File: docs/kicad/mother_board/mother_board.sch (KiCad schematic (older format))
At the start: 14 parts, among them J1 EXPR, J2 TFT_CONTROL, J3 TFT_DATA, J4 SERIAL, J5 LEDS, J6 ROTARY12, J7 ROTARY34, J8 SW_OUT, J9 SW_IN, U1 myTeensy3.6

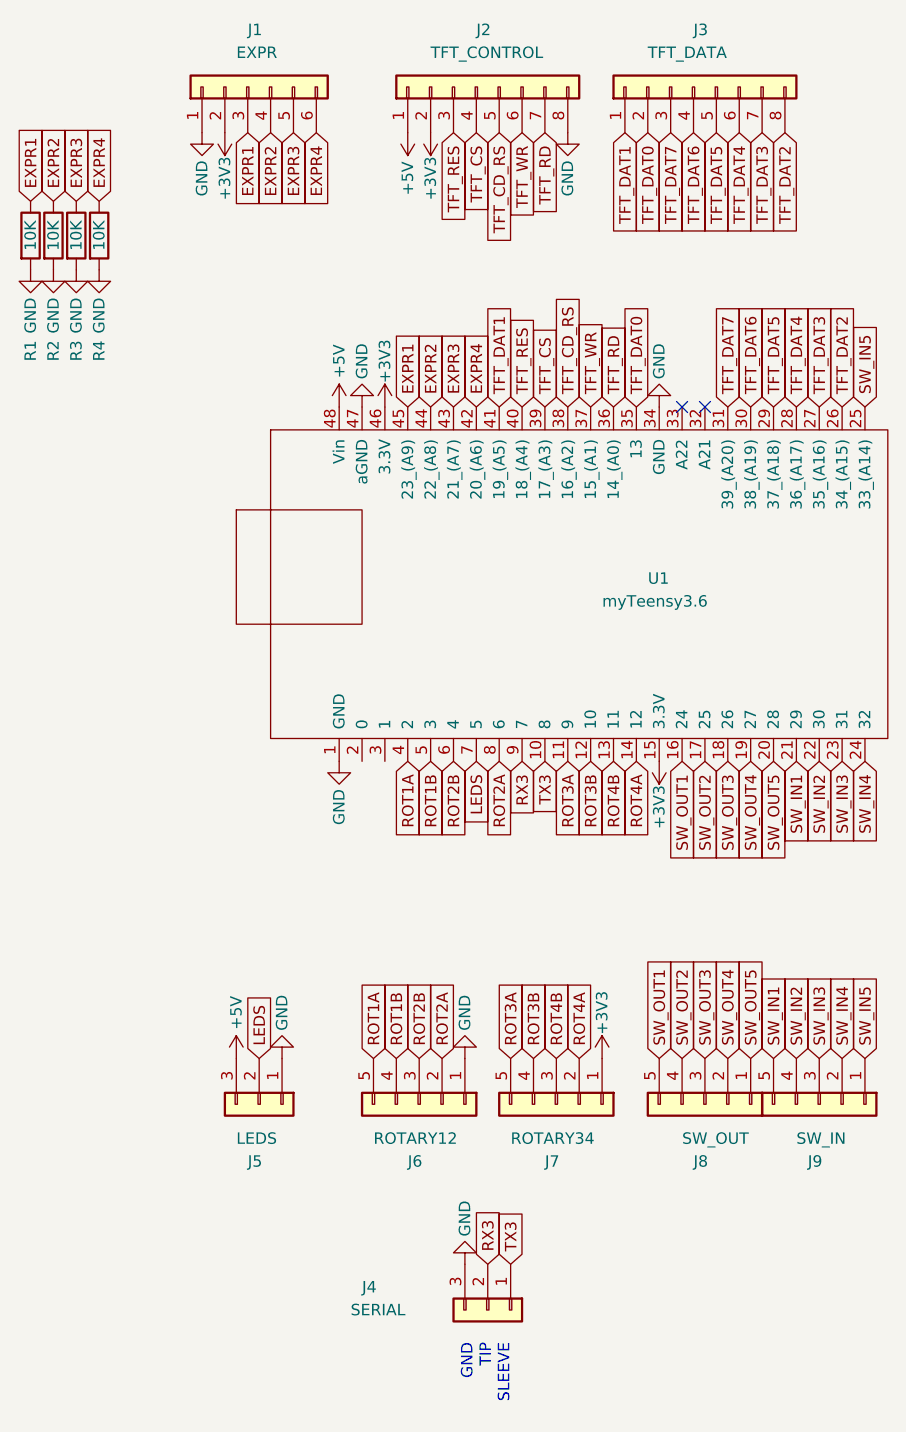
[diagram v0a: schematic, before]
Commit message: start MAKE NEW motherboard and display_connector FOR olds TeensyExprssion box with TE2 code
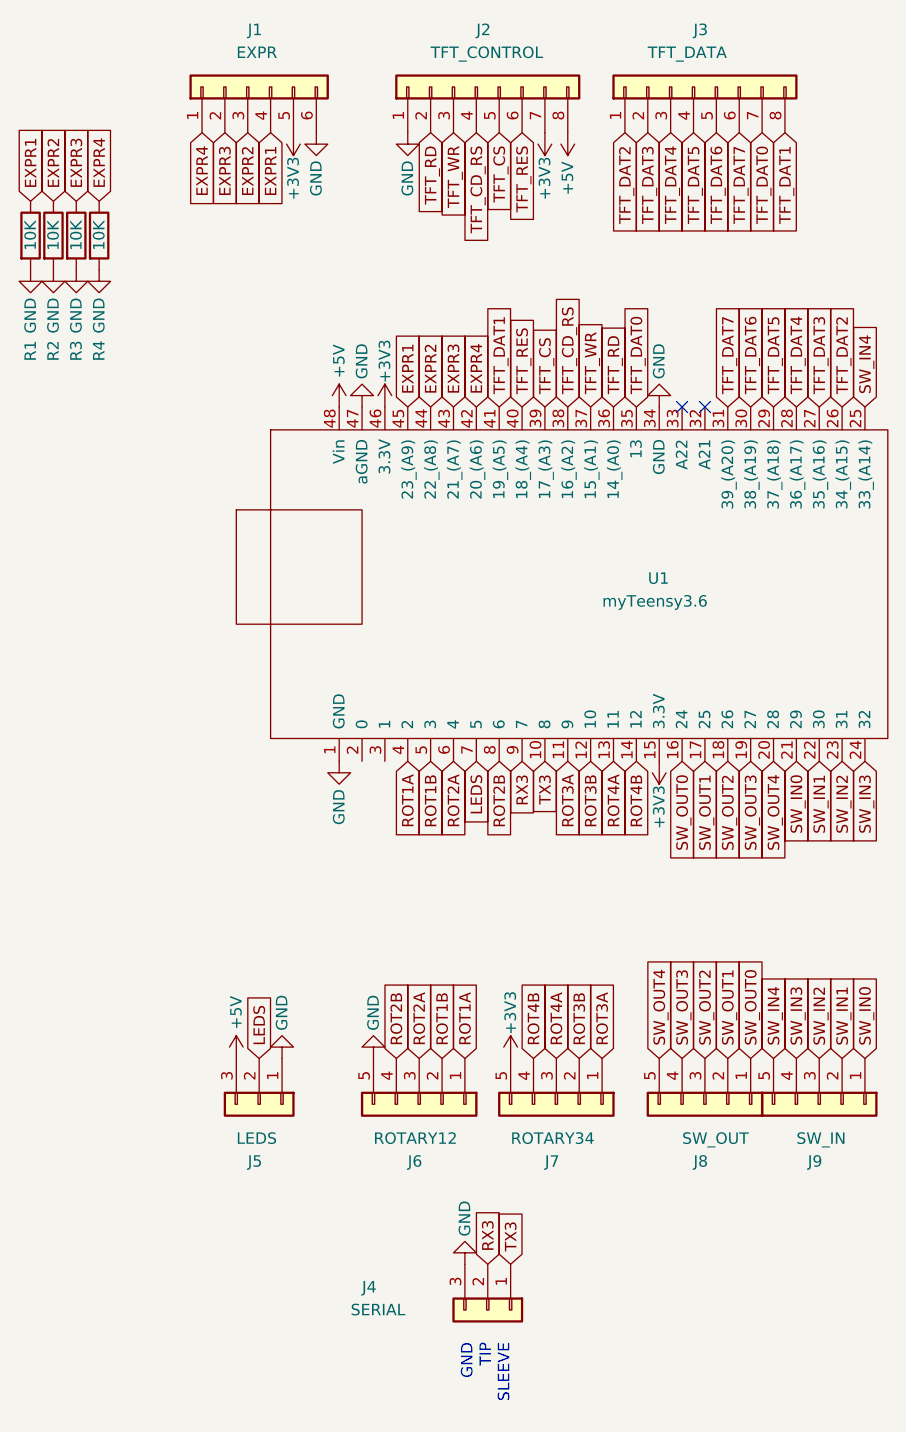
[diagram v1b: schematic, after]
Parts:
- J1: footprint 0_my_footprints:myJSTx06 -> 0_my_footprints:myPinSocket_1x06
- J4, J5: footprint 0_my_footprints:myJSTx03 -> 0_my_footprints:myPinSocket_1x03
- J6, J7, J8, J9: footprint 0_my_footprints:myJSTx05 -> 0_my_footprints:myPinSocket_1x05
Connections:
- net +3V3: now also J1.5 (Pin_5), J2.7 (Pin_7), J7.5 (Pin_5); no longer J1.2 (Pin_2), J2.2 (Pin_2), J7.1 (Pin_1)
- net +5V: now also J2.8 (Pin_8); no longer J2.1 (Pin_1)
- net EXPR1: now also J1.4 (Pin_4); no longer J1.3 (Pin_3)
- net EXPR2: now also J1.3 (Pin_3); no longer J1.4 (Pin_4)
- net EXPR3: now also J1.2 (Pin_2); no longer J1.5 (Pin_5)
- net EXPR4: now also J1.1 (Pin_1); no longer J1.6 (Pin_6)
- net GND: now also J1.6 (Pin_6), J2.1 (Pin_1), J6.5 (Pin_5); no longer J1.1 (Pin_1), J2.8 (Pin_8), J6.1 (Pin_1)
- net ROT1A: now also J6.1 (Pin_1); no longer J6.5 (Pin_5)
- net ROT1B: now also J6.2 (Pin_2); no longer J6.4 (Pin_4)
- net ROT2A: now also J6.3 (Pin_3), U1.6 (4); no longer J6.2 (Pin_2), U1.8 (6)
- net ROT2B: now also J6.4 (Pin_4), U1.8 (6); no longer J6.3 (Pin_3), U1.6 (4)
- net ROT3A: now also J7.1 (Pin_1); no longer J7.5 (Pin_5)
- net ROT3B: now also J7.2 (Pin_2); no longer J7.4 (Pin_4)
- net ROT4A: now also J7.3 (Pin_3), U1.13 (11); no longer J7.2 (Pin_2), U1.14 (12)
- net ROT4B: now also J7.4 (Pin_4), U1.14 (12); no longer J7.3 (Pin_3), U1.13 (11)
- net SW_IN1: now also J9.2 (Pin_2), U1.22 (30); no longer J9.5 (Pin_5), U1.21 (29)
- net SW_IN2: now also J9.3 (Pin_3), U1.23 (31); no longer J9.4 (Pin_4), U1.22 (30)
- net SW_IN3: now also J9.4 (Pin_4), U1.24 (32); no longer J9.3 (Pin_3), U1.23 (31)
- net SW_IN4: now also J9.5 (Pin_5), U1.25 (33_(A14)); no longer J9.2 (Pin_2), U1.24 (32)
- net SW_OUT1: now also J8.2 (Pin_2), U1.17 (25); no longer J8.5 (Pin_5), U1.16 (24)
- net SW_OUT2: now also J8.3 (Pin_3), U1.18 (26); no longer J8.4 (Pin_4), U1.17 (25)
- net SW_OUT3: now also J8.4 (Pin_4), U1.19 (27); no longer J8.3 (Pin_3), U1.18 (26)
- net SW_OUT4: now also J8.5 (Pin_5), U1.20 (28); no longer J8.2 (Pin_2), U1.19 (27)
- net TFT_CD_RS: now also J2.4 (Pin_4); no longer J2.5 (Pin_5)
- net TFT_CS: now also J2.5 (Pin_5); no longer J2.4 (Pin_4)
- net TFT_DAT0: now also J3.7 (Pin_7); no longer J3.2 (Pin_2)
- net TFT_DAT1: now also J3.8 (Pin_8); no longer J3.1 (Pin_1)
- net TFT_DAT2: now also J3.1 (Pin_1); no longer J3.8 (Pin_8)
- net TFT_DAT3: now also J3.2 (Pin_2); no longer J3.7 (Pin_7)
- net TFT_DAT4: now also J3.3 (Pin_3); no longer J3.6 (Pin_6)
- net TFT_DAT5: now also J3.4 (Pin_4); no longer J3.5 (Pin_5)
- net TFT_DAT6: now also J3.5 (Pin_5); no longer J3.4 (Pin_4)
- net TFT_DAT7: now also J3.6 (Pin_6); no longer J3.3 (Pin_3)
- net TFT_RD: now also J2.2 (Pin_2); no longer J2.7 (Pin_7)
- net TFT_RES: now also J2.6 (Pin_6); no longer J2.3 (Pin_3)
- net TFT_WR: now also J2.3 (Pin_3); no longer J2.6 (Pin_6)
- net SW_IN5 renamed SW_IN0
- net SW_IN0: now also U1.21 (29); no longer U1.25 (33_(A14))
- net SW_OUT5 renamed SW_OUT0
- net SW_OUT0: now also U1.16 (24); no longer U1.20 (28)
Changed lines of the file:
@@
 F 0 "J5" V 4250 5700 50  0000 L CNN
 F 1 "LEDS" V 4150 5650 50  0000 L CNN
-F 2 "0_my_footprints:myJSTx03" H 4000 5750 50  0001 C CNN
+F 2 "0_my_footprints:myPinSocket_1x03" H 4000 5750 50  0001 C CNN
 F 3 "~" H 4000 5750 50  0001 C CNN
 	1    4000 5750
@@
 F 0 "J6" V 4950 5700 50  0000 L CNN
 F 1 "ROTARY12" V 4850 5550 50  0000 L CNN
-F 2 "0_my_footprints:myJSTx05" H 4700 5750 50  0001 C CNN
+F 2 "0_my_footprints:myPinSocket_1x05" H 4700 5750 50  0001 C CNN
 F 3 "~" H 4700 5750 50  0001 C CNN
 	1    4700 5750
@@
 F 0 "J1" V 4200 1300 50  0000 R CNN
 F 1 "EXPR" V 4100 1350 50  0000 R CNN
-F 2 "0_my_footprints:myJSTx06" H 3950 1300 50  0001 C CNN
+F 2 "0_my_footprints:myPinSocket_1x06" H 3950 1300 50  0001 C CNN
 F 3 "~" H 3950 1300 50  0001 C CNN
 	1    3950 1300
@@
 F 0 "J7" V 5550 5700 50  0000 L CNN
 F 1 "ROTARY34" V 5450 5550 50  0000 L CNN
-F 2 "0_my_footprints:myJSTx05" H 5300 5750 50  0001 C CNN
+F 2 "0_my_footprints:myPinSocket_1x05" H 5300 5750 50  0001 C CNN
 F 3 "~" H 5300 5750 50  0001 C CNN
 	1    5300 5750
@@
 F 0 "J8" V 6200 5700 50  0000 L CNN
 F 1 "SW_OUT" V 6100 5650 50  0000 L CNN
-F 2 "0_my_footprints:myJSTx05" H 5950 5750 50  0001 C CNN
+F 2 "0_my_footprints:myPinSocket_1x05" H 5950 5750 50  0001 C CNN
 F 3 "~" H 5950 5750 50  0001 C CNN
 	1    5950 5750
@@
 F 0 "J9" V 6700 5700 50  0000 L CNN
 F 1 "SW_IN" V 6600 5650 50  0000 L CNN
-F 2 "0_my_footprints:myJSTx05" H 6450 5750 50  0001 C CNN
+F 2 "0_my_footprints:myPinSocket_1x05" H 6450 5750 50  0001 C CNN
 F 3 "~" H 6450 5750 50  0001 C CNN
 	1    6450 5750
@@
 F 0 "J4" V 4900 6100 50  0000 L CNN
 F 1 "SERIAL" V 5000 6050 50  0000 L CNN
-F 2 "0_my_footprints:myJSTx03" H 5000 6650 50  0001 C CNN
+F 2 "0_my_footprints:myPinSocket_1x03" H 5000 6650 50  0001 C CNN
 F 3 "~" H 5000 6650 50  0001 C CNN
 	1    5000 6650
@@
 L power:+3V3 #PWR016
 U 1 1 64C9FDB5
-P 5500 5550
-F 0 "#PWR016" H 5500 5400 50  0001 C CNN
-F 1 "+3V3" V 5500 5750 50  0000 C CNN
-F 2 "" H 5500 5550 50  0001 C CNN
-F 3 "" H 5500 5550 50  0001 C CNN
-	1    5500 5550
+P 5100 5550
+F 0 "#PWR016" H 5100 5400 50  0001 C CNN
+F 1 "+3V3" V 5100 5750 50  0000 C CNN
+F 2 "" H 5100 5550 50  0001 C CNN
+F 3 "" H 5100 5550 50  0001 C CNN
+	1    5100 5550
 	1    0    0    -1
 $EndComp
@@
 L power:GND #PWR015
 U 1 1 64CA12B5
-P 4900 5550
-F 0 "#PWR015" H 4900 5300 50  0001 C CNN
-F 1 "GND" V 4900 5350 50  0000 C CNN
-F 2 "" H 4900 5550 50  0001 C CNN
-F 3 "" H 4900 5550 50  0001 C CNN
-	1    4900 5550
+P 4500 5550
+F 0 "#PWR015" H 4500 5300 50  0001 C CNN
+F 1 "GND" V 4500 5350 50  0000 C CNN
+F 2 "" H 4500 5550 50  0001 C CNN
+F 3 "" H 4500 5550 50  0001 C CNN
+	1    4500 5550
 	-1   0    0    1
 $EndComp
@@
 	-1   0    0    1
 $EndComp
-Text GLabel 4950 4250 3    50   Input ~ 0
-LEDS
 Text GLabel 4650 4250 3    50   Input ~ 0
 ROT1A
@@
 ROT1B
 Text GLabel 4850 4250 3    50   Input ~ 0
-ROT2B
-Text GLabel 5050 4250 3    50   Input ~ 0
 ROT2A
 Text GLabel 5150 4250 3    50   Input ~ 0
@@
 Text GLabel 5450 4250 3    50   Input ~ 0
 ROT3B
+Text GLabel 5650 4250 3    50   Input ~ 0
+ROT4B
 Text GLabel 5550 4250 3    50   Input ~ 0
+ROT4A
+Text GLabel 4900 5550 1    50   Input ~ 0
+ROT1A
+Text GLabel 4800 5550 1    50   Input ~ 0
+ROT1B
+Text GLabel 4600 5550 1    50   Input ~ 0
+ROT2B
+Text GLabel 4700 5550 1    50   Input ~ 0
+ROT2A
+Text GLabel 5500 5550 1    50   Input ~ 0
+ROT3A
+Text GLabel 5400 5550 1    50   Input ~ 0
+ROT3B
+Text GLabel 5200 5550 1    50   Input ~ 0
 ROT4B
-Text GLabel 5650 4250 3    50   Input ~ 0
-ROT4A
-Text GLabel 4500 5550 1    50   Input ~ 0
-ROT1A
-Text GLabel 4600 5550 1    50   Input ~ 0
-ROT1B
-Text GLabel 4700 5550 1    50   Input ~ 0
-ROT2B
-Text GLabel 4800 5550 1    50   Input ~ 0
-ROT2A
-Text GLabel 5100 5550 1    50   Input ~ 0
-ROT3A
-Text GLabel 5200 5550 1    50   Input ~ 0
-ROT3B
 Text GLabel 5300 5550 1    50   Input ~ 0
-ROT4B
-Text GLabel 5400 5550 1    50   Input ~ 0
 ROT4A
 Text GLabel 5850 4250 3    50   Input ~ 0
+SW_OUT0
+Text GLabel 5950 4250 3    50   Input ~ 0
 SW_OUT1
-Text GLabel 5950 4250 3    50   Input ~ 0
+Text GLabel 6050 4250 3    50   Input ~ 0
 SW_OUT2
-Text GLabel 6050 4250 3    50   Input ~ 0
+Text GLabel 6150 4250 3    50   Input ~ 0
 SW_OUT3
-Text GLabel 6150 4250 3    50   Input ~ 0
+Text GLabel 6250 4250 3    50   Input ~ 0
 SW_OUT4
-Text GLabel 6250 4250 3    50   Input ~ 0
-SW_OUT5
 Text GLabel 6350 4250 3    50   Input ~ 0
+SW_IN0
+Text GLabel 6450 4250 3    50   Input ~ 0
 SW_IN1
-Text GLabel 6450 4250 3    50   Input ~ 0
+Text GLabel 6550 4250 3    50   Input ~ 0
 SW_IN2
-Text GLabel 6550 4250 3    50   Input ~ 0
+Text GLabel 6650 4250 3    50   Input ~ 0
 SW_IN3
-Text GLabel 6650 4250 3    50   Input ~ 0
+Text GLabel 6650 2700 1    50   Input ~ 0
 SW_IN4
-Text GLabel 6650 2700 1    50   Input ~ 0
-SW_IN5
+Text GLabel 6050 5550 1    50   Input ~ 0
+SW_OUT1
+Text GLabel 5950 5550 1    50   Input ~ 0
+SW_OUT2
+Text GLabel 5850 5550 1    50   Input ~ 0
+SW_OUT3
 Text GLabel 5750 5550 1    50   Input ~ 0
-SW_OUT1
-Text GLabel 5850 5550 1    50   Input ~ 0
-SW_OUT2
-Text GLabel 5950 5550 1    50   Input ~ 0
-SW_OUT3
-Text GLabel 6050 5550 1    50   Input ~ 0
 SW_OUT4
 Text GLabel 6150 5550 1    50   Input ~ 0
-SW_OUT5
+SW_OUT0
+Text GLabel 6550 5550 1    50   Input ~ 0
+SW_IN1
+Text GLabel 6450 5550 1    50   Input ~ 0
+SW_IN2
+Text GLabel 6350 5550 1    50   Input ~ 0
+SW_IN3
 Text GLabel 6250 5550 1    50   Input ~ 0
-SW_IN1
-Text GLabel 6350 5550 1    50   Input ~ 0
-SW_IN2
-Text GLabel 6450 5550 1    50   Input ~ 0
-SW_IN3
-Text GLabel 6550 5550 1    50   Input ~ 0
 SW_IN4
 Text GLabel 6650 5550 1    50   Input ~ 0
-SW_IN5
+SW_IN0
 $Comp
 L power:GND #PWR01
 U 1 1 64CFCC09
-P 3750 1500
-F 0 "#PWR01" H 3750 1250 50  0001 C CNN
-F 1 "GND" V 3750 1300 50  0000 C CNN
-F 2 "" H 3750 1500 50  0001 C CNN
-F 3 "" H 3750 1500 50  0001 C CNN
-	1    3750 1500
-	1    0    0    -1
+P 4250 1500
+F 0 "#PWR01" H 4250 1250 50  0001 C CNN
+F 1 "GND" V 4250 1300 50  0000 C CNN
+F 2 "" H 4250 1500 50  0001 C CNN
+F 3 "" H 4250 1500 50  0001 C CNN
+	1    4250 1500
+	-1   0    0    -1
 $EndComp
 $Comp
@@
 	1    0    0    -1
 $EndComp
+Text GLabel 4050 1500 3    50   Input ~ 0
+EXPR1
 Text GLabel 3950 1500 3    50   Input ~ 0
-EXPR1
-Text GLabel 4050 1500 3    50   Input ~ 0
 EXPR2
-Text GLabel 4150 1500 3    50   Input ~ 0
+Text GLabel 3850 1500 3    50   Input ~ 0
 EXPR3
-Text GLabel 4250 1500 3    50   Input ~ 0
+Text GLabel 3750 1500 3    50   Input ~ 0
 EXPR4
 Text GLabel 4650 2700 1    50   Input ~ 0
@@
 L power:+5V #PWR02
 U 1 1 64D14F5D
+P 5350 1500
+F 0 "#PWR02" H 5350 1350 50  0001 C CNN
+F 1 "+5V" V 5350 1700 50  0000 C CNN
+F 2 "" H 5350 1500 50  0001 C CNN
+F 3 "" H 5350 1500 50  0001 C CNN
+	1    5350 1500
+	1    0    0    1
+$EndComp
+$Comp
+L power:GND #PWR04
+U 1 1 64D19F15
 P 4650 1500
-F 0 "#PWR02" H 4650 1350 50  0001 C CNN
-F 1 "+5V" V 4650 1700 50  0000 C CNN
+F 0 "#PWR04" H 4650 1250 50  0001 C CNN
+F 1 "GND" V 4650 1300 50  0000 C CNN
 F 2 "" H 4650 1500 50  0001 C CNN
 F 3 "" H 4650 1500 50  0001 C CNN
 	1    4650 1500
-	-1   0    0    1
-$EndComp
-$Comp
-L power:GND #PWR04
-U 1 1 64D19F15
-P 5350 1500
-F 0 "#PWR04" H 5350 1250 50  0001 C CNN
-F 1 "GND" V 5350 1300 50  0000 C CNN
-F 2 "" H 5350 1500 50  0001 C CNN
-F 3 "" H 5350 1500 50  0001 C CNN
-	1    5350 1500
-	1    0    0    -1
-$EndComp
+	-1   0    0    -1
+$EndComp
+Text GLabel 5150 1500 3    50   Input ~ 0
+TFT_RES
+Text GLabel 5050 1500 3    50   Input ~ 0
+TFT_CS
+Text GLabel 4950 1500 3    50   Input ~ 0
+TFT_CD_RS
 Text GLabel 4850 1500 3    50   Input ~ 0
-TFT_RES
-Text GLabel 4950 1500 3    50   Input ~ 0
-TFT_CS
-Text GLabel 5050 1500 3    50   Input ~ 0
-TFT_CD_RS
-Text GLabel 5150 1500 3    50   Input ~ 0
 TFT_WR
-Text GLabel 5250 1500 3    50   Input ~ 0
+Text GLabel 4750 1500 3    50   Input ~ 0
 TFT_RD
+Text GLabel 6300 1500 3    50   Input ~ 0
+TFT_DAT1
+Text GLabel 6200 1500 3    50   Input ~ 0
+TFT_DAT0
+Text GLabel 6100 1500 3    50   Input ~ 0
+TFT_DAT7
+Text GLabel 6000 1500 3    50   Input ~ 0
+TFT_DAT6
+Text GLabel 5900 1500 3    50   Input ~ 0
+TFT_DAT5
+Text GLabel 5800 1500 3    50   Input ~ 0
+TFT_DAT4
+Text GLabel 5700 1500 3    50   Input ~ 0
+TFT_DAT3
 Text GLabel 5600 1500 3    50   Input ~ 0
-TFT_DAT1
-Text GLabel 5700 1500 3    50   Input ~ 0
-TFT_DAT0
-Text GLabel 5800 1500 3    50   Input ~ 0
-TFT_DAT7
-Text GLabel 5900 1500 3    50   Input ~ 0
-TFT_DAT6
-Text GLabel 6000 1500 3    50   Input ~ 0
-TFT_DAT5
-Text GLabel 6100 1500 3    50   Input ~ 0
-TFT_DAT4
-Text GLabel 6200 1500 3    50   Input ~ 0
-TFT_DAT3
-Text GLabel 6300 1500 3    50   Input ~ 0
 TFT_DAT2
 Text GLabel 5150 2700 1    50   Input ~ 0
@@
 L power:+3V3 #PWR03
 U 1 1 64D171C2
-P 4750 1500
-F 0 "#PWR03" H 4750 1350 50  0001 C CNN
-F 1 "+3V3" V 4750 1700 50  0000 C CNN
-F 2 "" H 4750 1500 50  0001 C CNN
-F 3 "" H 4750 1500 50  0001 C CNN
-	1    4750 1500
-	-1   0    0    1
+P 5250 1500
+F 0 "#PWR03" H 5250 1350 50  0001 C CNN
+F 1 "+3V3" V 5250 1700 50  0000 C CNN
+F 2 "" H 5250 1500 50  0001 C CNN
+F 3 "" H 5250 1500 50  0001 C CNN
+	1    5250 1500
+	1    0    0    1
 $EndComp
 $Comp
 L power:+3V3 #PWR06
 U 1 1 64D07CE1
-P 3850 1500
-F 0 "#PWR06" H 3850 1350 50  0001 C CNN
-F 1 "+3V3" V 3850 1700 50  0000 C CNN
-F 2 "" H 3850 1500 50  0001 C CNN
-F 3 "" H 3850 1500 50  0001 C CNN
-	1    3850 1500
-	-1   0    0    1
+P 4150 1500
+F 0 "#PWR06" H 4150 1350 50  0001 C CNN
+F 1 "+3V3" V 4150 1700 50  0000 C CNN
+F 2 "" H 4150 1500 50  0001 C CNN
+F 3 "" H 4150 1500 50  0001 C CNN
+	1    4150 1500
+	1    0    0    1
 $EndComp
 Text GLabel 3000 1800 1    50   Input ~ 0
@@
 	1    0    0    -1
 $EndComp
+Text GLabel 5050 4250 3    50   Input ~ 0
+ROT2B
+Text GLabel 4950 4250 3    50   Input ~ 0
+LEDS
 $EndSCHEMATC
